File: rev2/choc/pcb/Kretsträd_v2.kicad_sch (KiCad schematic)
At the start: 49 parts, among them J1 Conn_01x02_Female, J2 Conn_01x02_Female, J3 Conn_01x02_Female, J4 Conn_01x02_Female, SW1 ${REFERENCE}, SW10 ${REFERENCE}, SW11 ${REFERENCE}, SW12 ${REFERENCE}, SW13 ${REFERENCE}, SW14 ${REFERENCE}, SW15 ${REFERENCE}, SW16 ${REFERENCE}, SW17 ${REFERENCE}, SW2 ${REFERENCE}, SW3 ${REFERENCE}, SW4 ${REFERENCE}, SW5 ${REFERENCE}, SW6 ${REFERENCE}, SW7 ${REFERENCE}, SW8 ${REFERENCE}, SW9 ${REFERENCE}, U1 SeeeduinoXIAO

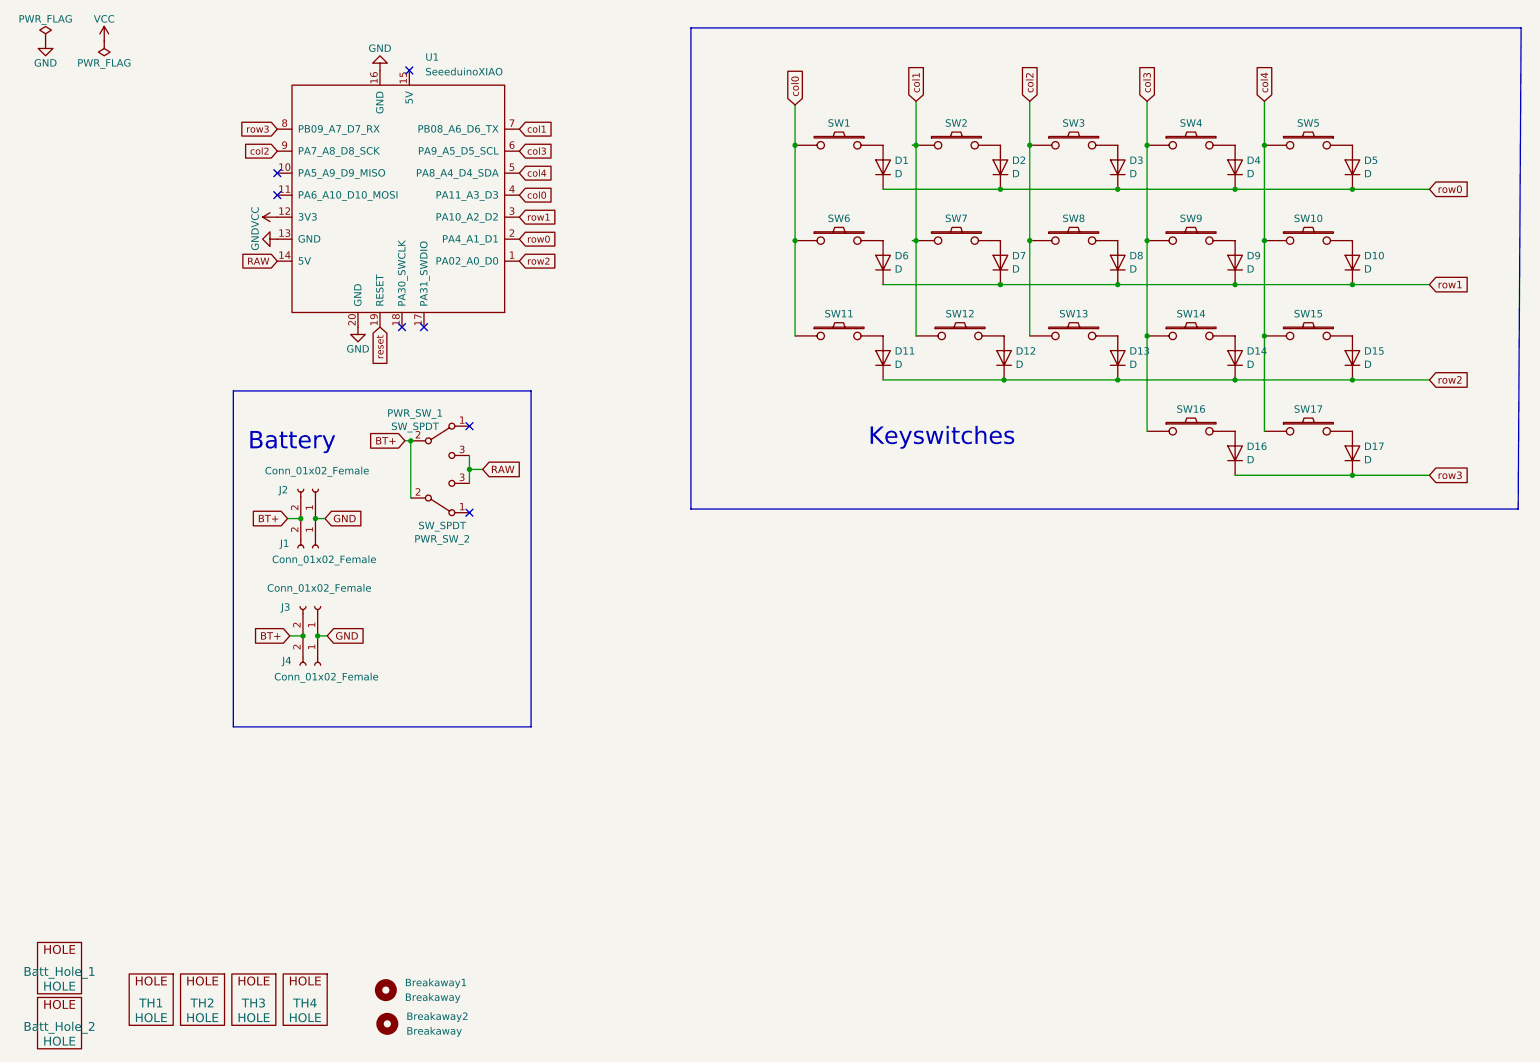
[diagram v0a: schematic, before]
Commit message: v2.1: pre-production iteration
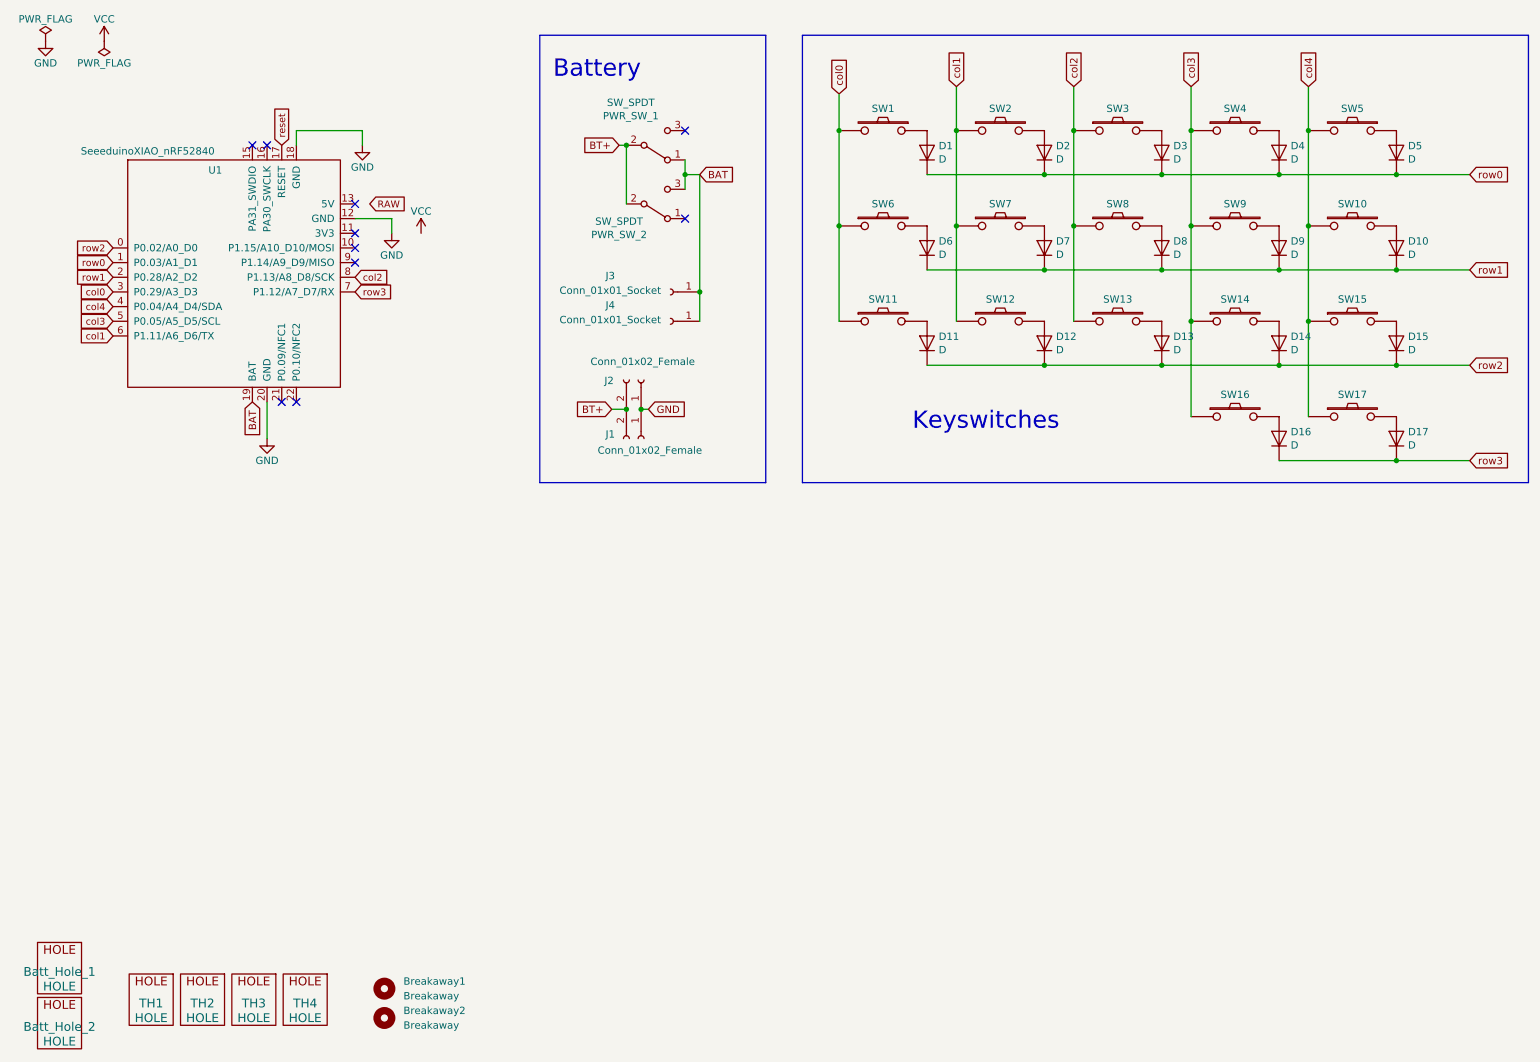
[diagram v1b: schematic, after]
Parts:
- removed J3, J4: Conn_01x02_Female, Connector_Molex:Molex_Panelmate_53780-0270_1x02-1MP_P1.25mm_Horizontal, symbol Connector:Conn_01x02_Female
- removed U1: SeeeduinoXIAO, jw_custom_footprints:Xiao THT jumper pad_big_hole_flipped, symbol Seeeduino XIAO:SeeeduinoXIAO
- added J3, J4: Conn_01x01_Socket, jw_custom_footprints:Pogopin_socket_1x01_1.00mm_vertical, symbol Connector:Conn_01x01_Socket
- added U1: SeeeduinoXIAO_nRF52840, jw_custom_footprints:Xiao_nRF52840_THT_jumper_1.55mm_hole, symbol jw_custom_symbols:SeeeduinoXIAO_nRF52840
- D1, D10, D11, D12, D13, D14, D15, D16, D17, D2, D3, D4, D5, D6, D7, D8, D9: footprint jw_custom_footprint:Diode_SOD123_THT_2 -> jw_custom_footprints:Diode_SOD123_THT_2
- SW1, SW10, SW11, SW12, SW13, SW14, SW15, SW16, SW17, SW2, SW3, SW4, SW5, SW6, SW7, SW8, SW9: footprint jw_custom_footprint:Kailh_Choc_PG1350_Hotswap_reversible -> jw_custom_footprints:Kailh_Choc_PG1350_v1+2_Hotswap_reversible
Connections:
- net GND: now also U1.12 (GND), U1.18 (GND), U1.20 (GND)
- net RAW: no longer PWR_SW_1.3 (C), PWR_SW_2.3 (C)
- net col0: now also U1.3 (P0.29/A3_D3)
- net col1: now also U1.6 (P1.11/A6_D6/TX)
- net col2: now also U1.8 (P1.13/A8_D8/SCK)
- net col3: now also U1.5 (P0.05/A5_D5/SCL)
- net col4: now also U1.4 (P0.04/A4_D4/SDA)
- net reset: now also U1.17 (RESET)
- net row0: now also U1.1 (P0.03/A1_D1)
- net row1: now also U1.2 (P0.28/A2_D2)
- net row2: now also U1.0 (P0.02/A0_D0)
- net row3: now also U1.7 (P1.12/A7_D7/RX)
- net BAT: now reaches PWR_SW_1.1 (A)
- net BAT: now also PWR_SW_2.3 (C), J3.1 (Pin_1), J4.1 (Pin_1), U1.19 (BAT)
- no-connect marks 7 -> 10
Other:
- moved on the sheet: Breakaway2, D1, D10, D11, D12, D13, D14, D15, D16, D17, D2, D3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
